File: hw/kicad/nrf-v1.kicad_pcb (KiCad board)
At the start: 2 copper layers, 21.1 x 23 mm, 32 parts, among them U1 TPS62732, U2 nRF51822, U3 SST25WF040B, U4 BMA280, U5 STSC1, U6 BAL-NRF01D3, X1 16MHz, X2 32.768kHz

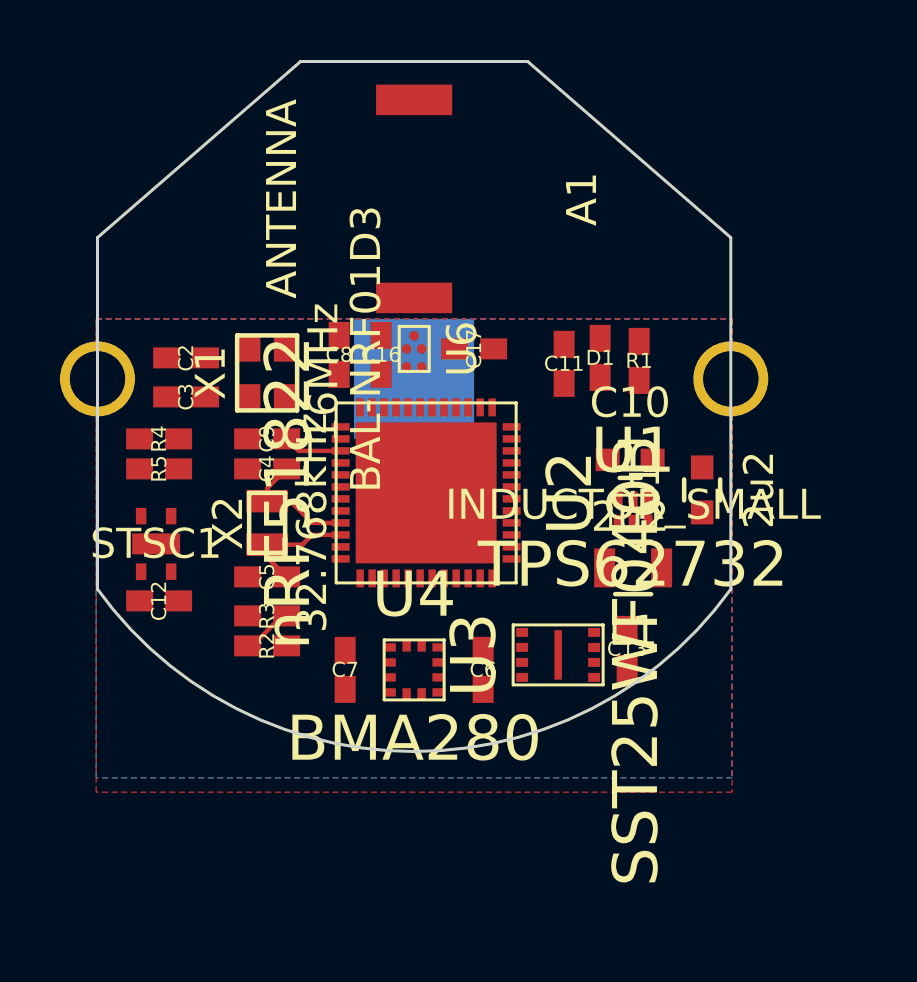
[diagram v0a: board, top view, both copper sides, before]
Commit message: PCB ready for 1st review
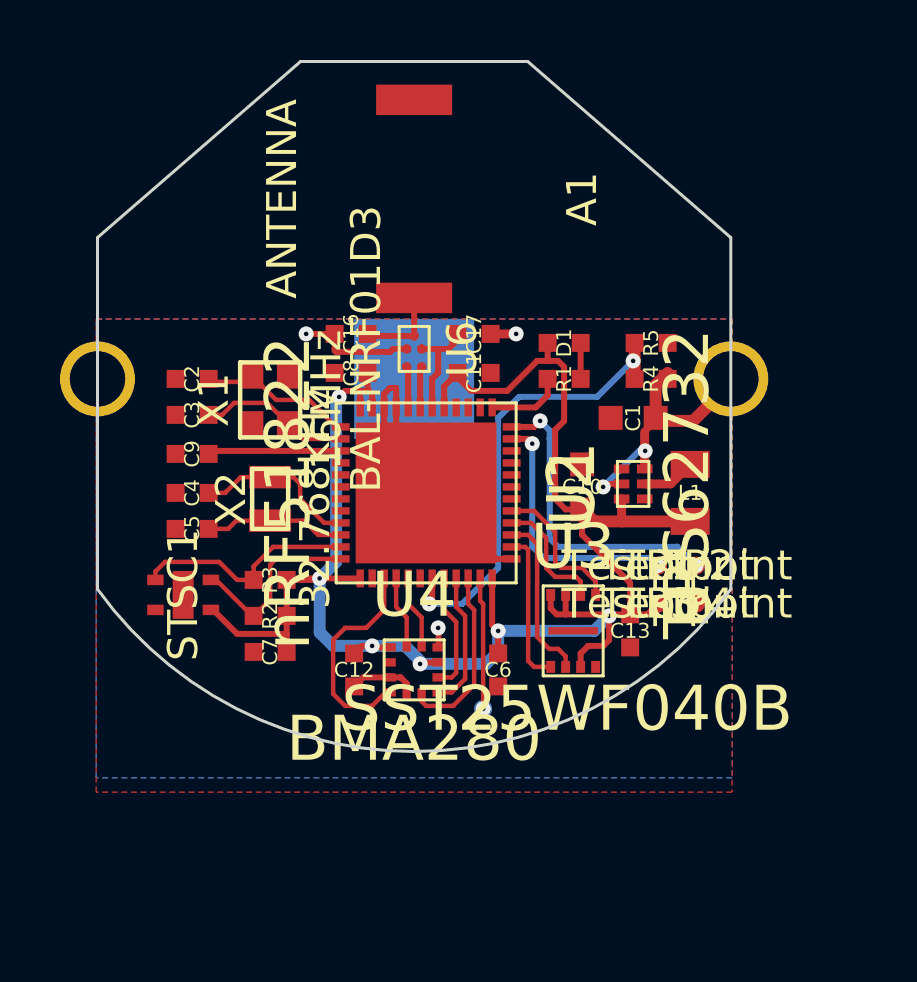
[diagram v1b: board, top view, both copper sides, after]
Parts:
- added TP1: Testpoint, project:TP_0.6, F.Cu at (108.1, 106.2)
- added TP2: Testpoint, project:TP_0.6, F.Cu at (109.4, 106.2)
- added TP3: Testpoint, project:TP_0.6, F.Cu at (108.1, 107.5)
- added TP4: Testpoint, project:TP_0.6, F.Cu at (109.4, 107.5)
- added TP5: Testpoint, project:TP_0.6, B.Cu at (102.3, 111.0)
- C1, C10: footprint Capacitors_SMD:C_0603 -> project:IPC-0603
- L1: footprint Resistors_SMD:R_0805 -> project:IPC-0805
- moved R5 16.9 mm to (107.9, 98.8), turned to 0 degrees
- moved R4 16.5 mm to (107.9, 100.0), turned to 180 degrees
- moved C12 6.89 mm to (98.0, 109.7), turned to 270 degrees
- moved C1 3.32 mm to (107.3, 101.3), turned to 180 degrees
- moved L1 3.14 mm to (109.2, 103.8), turned to 270 degrees
- moved C11 3.01 mm to (102.0, 99.8), turned to 0 degrees
- moved C5 2.97 mm to (92.6, 105.0)
- moved C4 2.62 mm to (92.6, 103.8)
- moved C7 2.57 mm to (95.2, 109.1), turned to 180 degrees
- moved R1 2.57 mm to (105.0, 100.0), turned to 180 degrees
- moved C9 2.55 mm to (92.6, 102.5)
- moved U5 1.92 mm to (92.3, 107.2), turned to 90 degrees
- moved C10 1.84 mm to (105.6, 103.6), turned to 90 degrees
- moved D1 1.30 mm to (105.0, 98.8), turned to 0 degrees
- moved C16 1.22 mm to (97.9, 98.5), turned to 180 degrees
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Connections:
- U1 pad 5: Net-(U1-Pad5) -> +BATT
- U2 pad 11: ~led -> bootloader
- U2 pad 14: Net-(U2-Pad14) -> spi0_cs_n
- U2 pad 15: Net-(U2-Pad15) -> spi0_miso
- U2 pad 16: Net-(U2-Pad16) -> spi0_sck
- U2 pad 17: Net-(U2-Pad17) -> spi0_mosi
- U2 pad 25: twi_sda -> ~led
- U2 pad 26: twi_scl -> Net-(U2-Pad26)
- U2 pad 41: spi0_cs_n -> Net-(U2-Pad41)
- U2 pad 42: spi0_miso -> Net-(U2-Pad42)
- U2 pad 43: spi0_sck -> Net-(U2-Pad43)
- U2 pad 44: spi0_mosi -> Net-(U2-Pad44)
- U2 pad 47: Net-(U2-Pad47) -> twi_sda
- U2 pad 48: Net-(U2-Pad48) -> twi_scl
- U2 pad 7: Net-(U2-Pad7) -> vbat_adc
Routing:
- net VDD: track 1.68 -> 64.0 mm, vias 0 -> 6
- net GND: track 0.00 -> 19.8 mm, vias 0 -> 3
- net vbat_adc: track 0.00 -> 15.5 mm, vias 0 -> 2
- net swclk: track 0.00 -> 10.4 mm, vias 0 -> 2
- net +BATT: track 0.00 -> 9.26 mm, vias 0 -> 2
- net swdio: track 0.00 -> 8.64 mm, vias 0 -> 2
- net twi_sda: track 0.00 -> 7.55 mm
- net spi1_cs_n: track 0.00 -> 7.20 mm
- net twi_scl: track 0.00 -> 6.28 mm
- net spi1_sck: track 0.00 -> 6.10 mm
- net spi0_miso: track 0.00 -> 5.64 mm
- net Net-(C2-Pad1): track 0.00 -> 5.21 mm
- net spi0_cs_n: track 0.00 -> 5.12 mm
- net Net-(C3-Pad1): track 0.00 -> 5.06 mm
- net spi0_mosi: track 0.00 -> 4.81 mm
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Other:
- net class Default: via_dia 0.3 -> 0.5
- rule via_min_size: 0.3 -> 0.5
